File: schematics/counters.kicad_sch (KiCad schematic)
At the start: 50 parts, among them Q1 S8050, U1 74HC14, U10 74HC390, U3 74HC86, U4 74HC4046, U5 74HC390, U6 74HC390, U7 74HC390, U8 LMC555xN, U9 74HC390

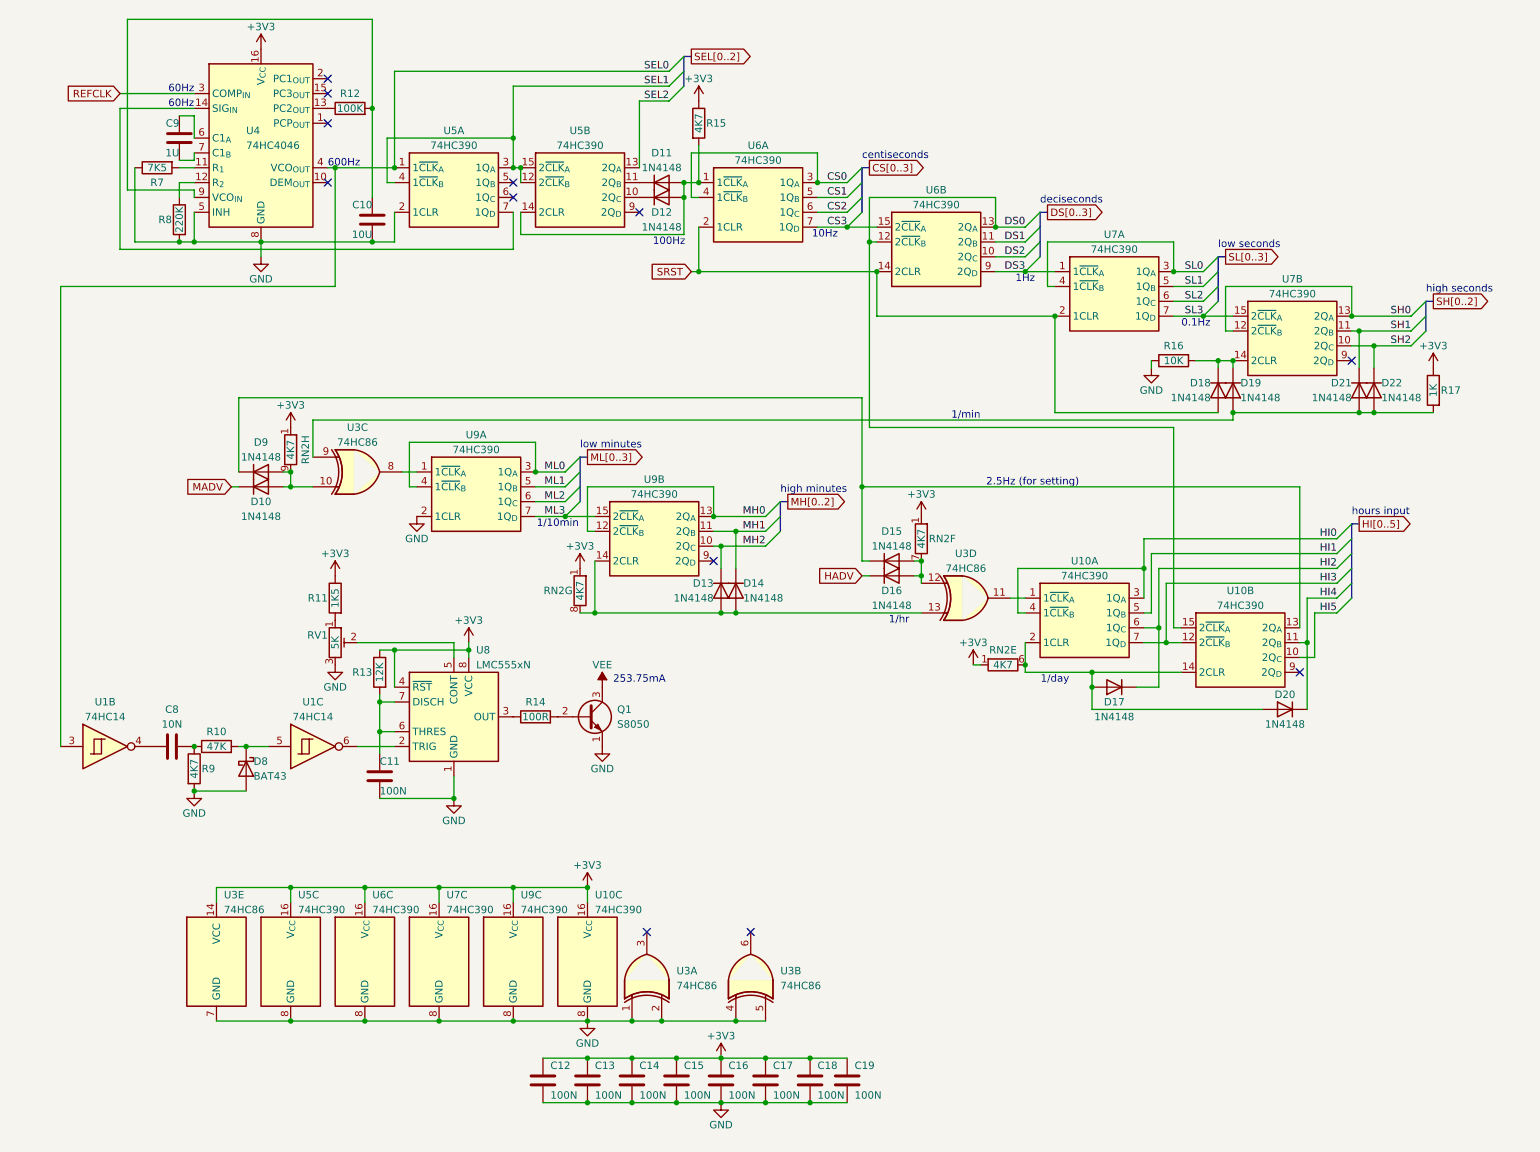
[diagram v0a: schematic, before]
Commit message: preliminary PCB design
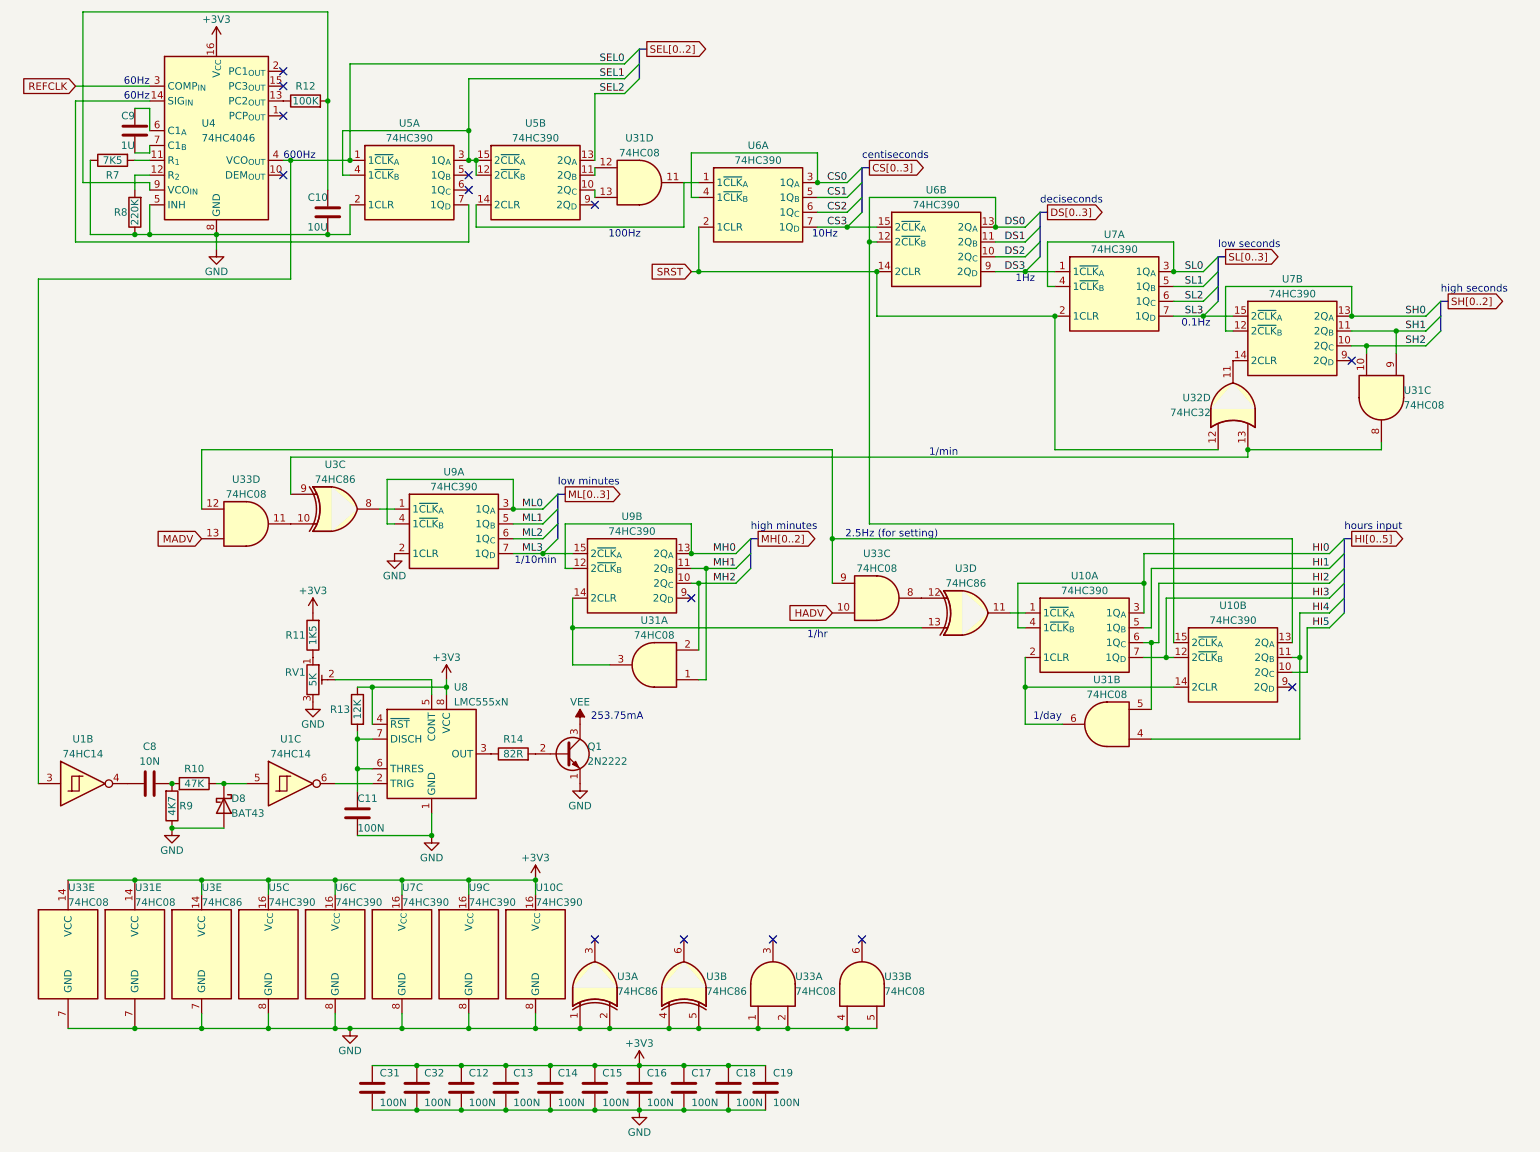
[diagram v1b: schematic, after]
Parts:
- removed D10, D11, D12, D13, D14, D15, D16, D17, D18, D19, D20, D21, D22, D9: 1N4148, Diode_THT:D_DO-35_SOD27_P7.62mm_Horizontal, symbol Diode:1N4148
- removed R15: 4K7, Resistor_THT:R_Axial_DIN0207_L6.3mm_D2.5mm_P7.62mm_Horizontal, symbol Device:R
- removed R16: 10K, Resistor_THT:R_Axial_DIN0207_L6.3mm_D2.5mm_P7.62mm_Horizontal, symbol Device:R
- removed R17: 1K, Resistor_THT:R_Axial_DIN0207_L6.3mm_D2.5mm_P7.62mm_Horizontal, symbol Device:R
- removed RN2: 4K7, Resistor_THT:R_Array_SIP9, symbol Device:R_Network08_Split
- added C31, C32: 100N, bvclock:THT_Cap, symbol Device:C
- added U31, U33: 74HC08, Package_DIP:DIP-14_W7.62mm, symbol 74xx:74LS08
- added U32: 74HC32, Package_DIP:DIP-14_W7.62mm, symbol 74xx:74LS32
- C10, C11, C12, C13, C14, C15, C16, C17, C18, C19, C8, C9: footprint Capacitor_THT:C_Disc_D5.1mm_W3.2mm_P5.00mm -> bvclock:THT_Cap
- D8: footprint Diode_THT:D_DO-35_SOD27_P7.62mm_Horizontal -> bvclock:THT_D_Vertical
- Q1: value S8050 -> 2N2222
- R10, R11, R12, R13, R7, R8, R9: footprint Resistor_THT:R_Axial_DIN0207_L6.3mm_D2.5mm_P7.62mm_Horizontal -> bvclock:THT_R_Vertical
- R14: value 100R -> 82R; footprint Resistor_THT:R_Axial_DIN0207_L6.3mm_D2.5mm_P7.62mm_Horizontal -> bvclock:THT_R_Vertical
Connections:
- net +3V3: now also R11.2, C31.1, C32.1, U31.14 (VCC), U33.14 (VCC); no longer R11.1
- net GND: now also R8.1, R9.1, C31.2, C32.2, U31.7 (GND), U33.1, U33.2, U33.4, U33.5, U33.7 (GND); no longer R8.2, R9.2
- net HADV: now also U33.10
- net HI2: now also U31.5
- net HI4: now also U31.4
- net MADV: now also U33.13
- net MH1: now also U31.1
- net MH2: now also U31.2
- net SH1: now also U31.9
- net SH2: now also U31.10
- net SRST: now also U32.12
- net at U3.10: now also U33.11
- net at U3.13, U9.14 (2CLR): now also U31.3
- net at U10.13 (2Q_{A}): now also U33.12, U33.9
- net at U3.12: now also U33.8
- net at U10.14 (2CLR), U10.2 (1CLR): now also U31.6
- net at U3.9: now also U31.8, U32.13
- net at RV1.1: now also R11.1; no longer R11.2
- net at D8.1 (K), U1.5: now also R10.1; no longer R10.2
- net at U7.14 (2CLR): now also U32.11
- net at U5.11 (2Q_{B}): now also U31.12
- net at U5.14 (2CLR), U6.1 (1~{CLK}_{A}): now also U31.11
- net at U4.12 (R_{2}): now also R8.2; no longer R8.1
- net at U5.10 (2Q_{C}): now also U31.13
- new net: C8.2, R10.2, R9.2
- no-connect marks 12 -> 14
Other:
- moved on the sheet: C10, C11, C12, C13, C14, C15, C16, C17, C18, C19, C8, C9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

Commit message: fixing DRC violations...
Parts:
- Q1: footprint Package_TO_SOT_THT:TO-92_HandSolder -> bvclock:TO-92_HandSolder
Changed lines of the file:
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@@
 			)
 		)
-		(property "Footprint" "Package_TO_SOT_THT:TO-92_HandSolder"
+		(property "Footprint" "bvclock:TO-92_HandSolder"
 			(at 107.95 135.89 0)
 			(hide yes)
